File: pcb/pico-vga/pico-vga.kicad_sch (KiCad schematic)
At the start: 42 parts, among them J1 DB15_Female_HighDensity, J2 Micro_SD_Card, J3 USB_A, J4 USB_A, J5 Conn_01x04_Male, J6 AudioJack3, J7 Conn_01x02_Male, J8 USB_A, J9 USB_A, Q1 DMP3099L-7, SW1 SW_Push, U1 Raspberry_Pi_Pico

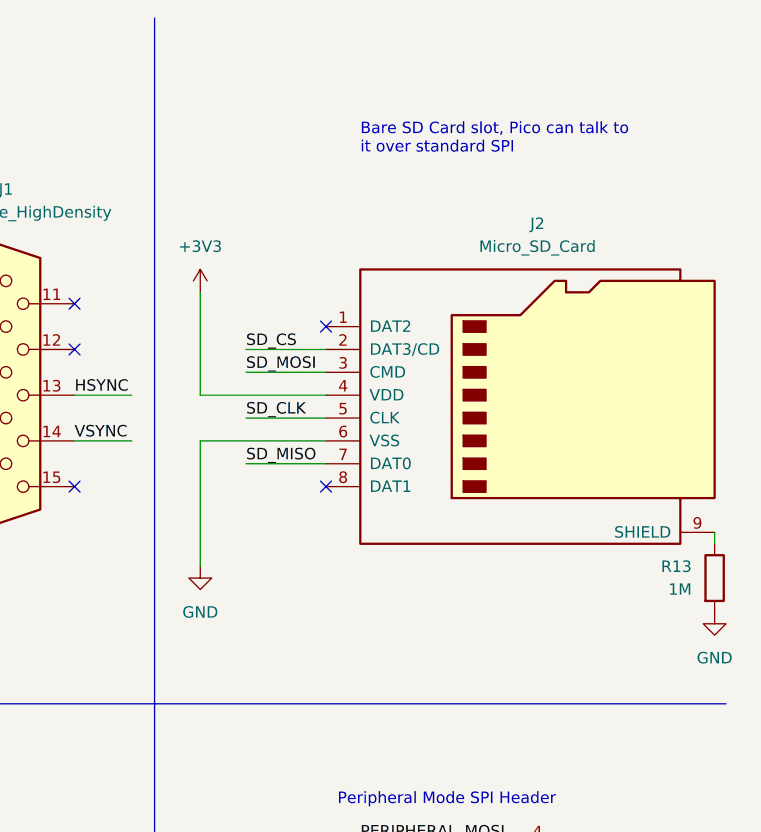
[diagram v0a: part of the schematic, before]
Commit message: PCB update and BOM
Remade the BOM so now you can just export to csv and throw it into digikey, makes it a lot easier. In making the BOM I realized some of my old parts were super expensive, so I redid some components
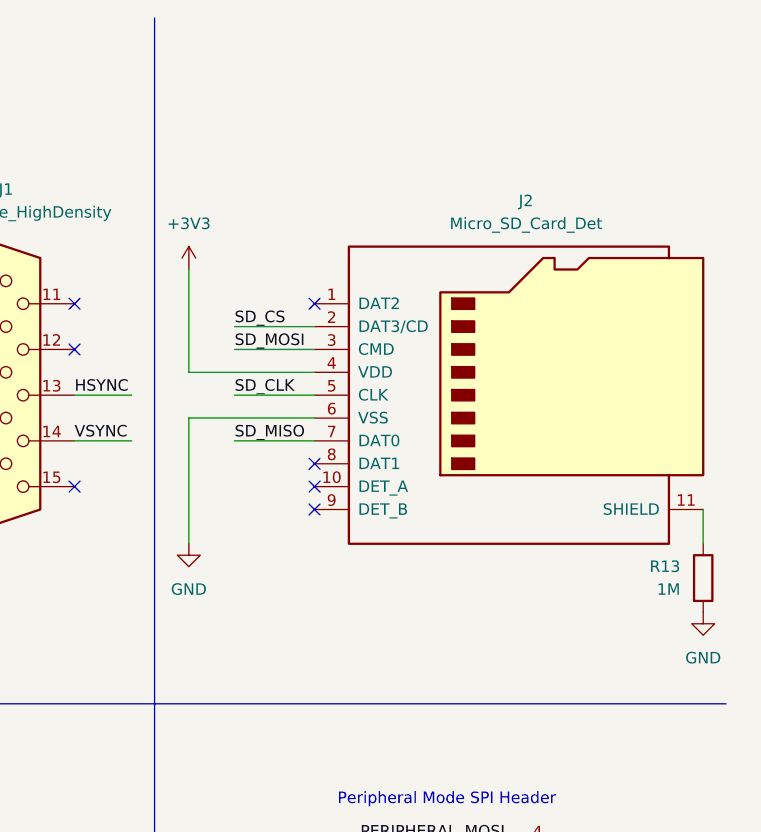
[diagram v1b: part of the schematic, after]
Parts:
- removed J2: Micro_SD_Card, Connector_Card:microSD_HC_Hirose_DM3AT-SF-PEJM5, symbol Connector:Micro_SD_Card
- added J2: Micro_SD_Card_Det, pico-vga:MEM2061-01-188-00-A_GCT, symbol Connector:Micro_SD_Card_Det
- J6: footprint Connector_Audio:Jack_3.5mm_CUI_SJ1-3533NG_Horizontal -> pico-vga:STX-3000_KYC
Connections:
- net +3V3: now also J2.4 (VDD)
- net GND: now also J2.6 (VSS)
- net SD_CLK: now also J2.5 (CLK)
- net SD_CS: now also J2.2 (DAT3/CD)
- net SD_MISO: now also J2.7 (DAT0)
- net SD_MOSI: now also J2.3 (CMD)
- net at R13.1: now also J2.11 (SHIELD)
- no-connect marks 17 -> 19
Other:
- note removed: "Bare SD Card slot, Pico can talk to it over standard SPI"
- moved on the sheet: R13
